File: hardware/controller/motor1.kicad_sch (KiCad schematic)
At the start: 55 parts, among them J10 Conn_01x01, J11 Conn_01x01, J12 Conn_02x03_Odd_Even, J9 Conn_01x01, Q10 AOD66406, Q11 AOD66406, Q12 AOD66406, Q13 AOD66406, Q8 AOD66406, Q9 AOD66406, U14 LM2105D, U15 MCP6541, U16 LM2105D, U17 MCP6541, U18 LM2105D, U19 MCP6541

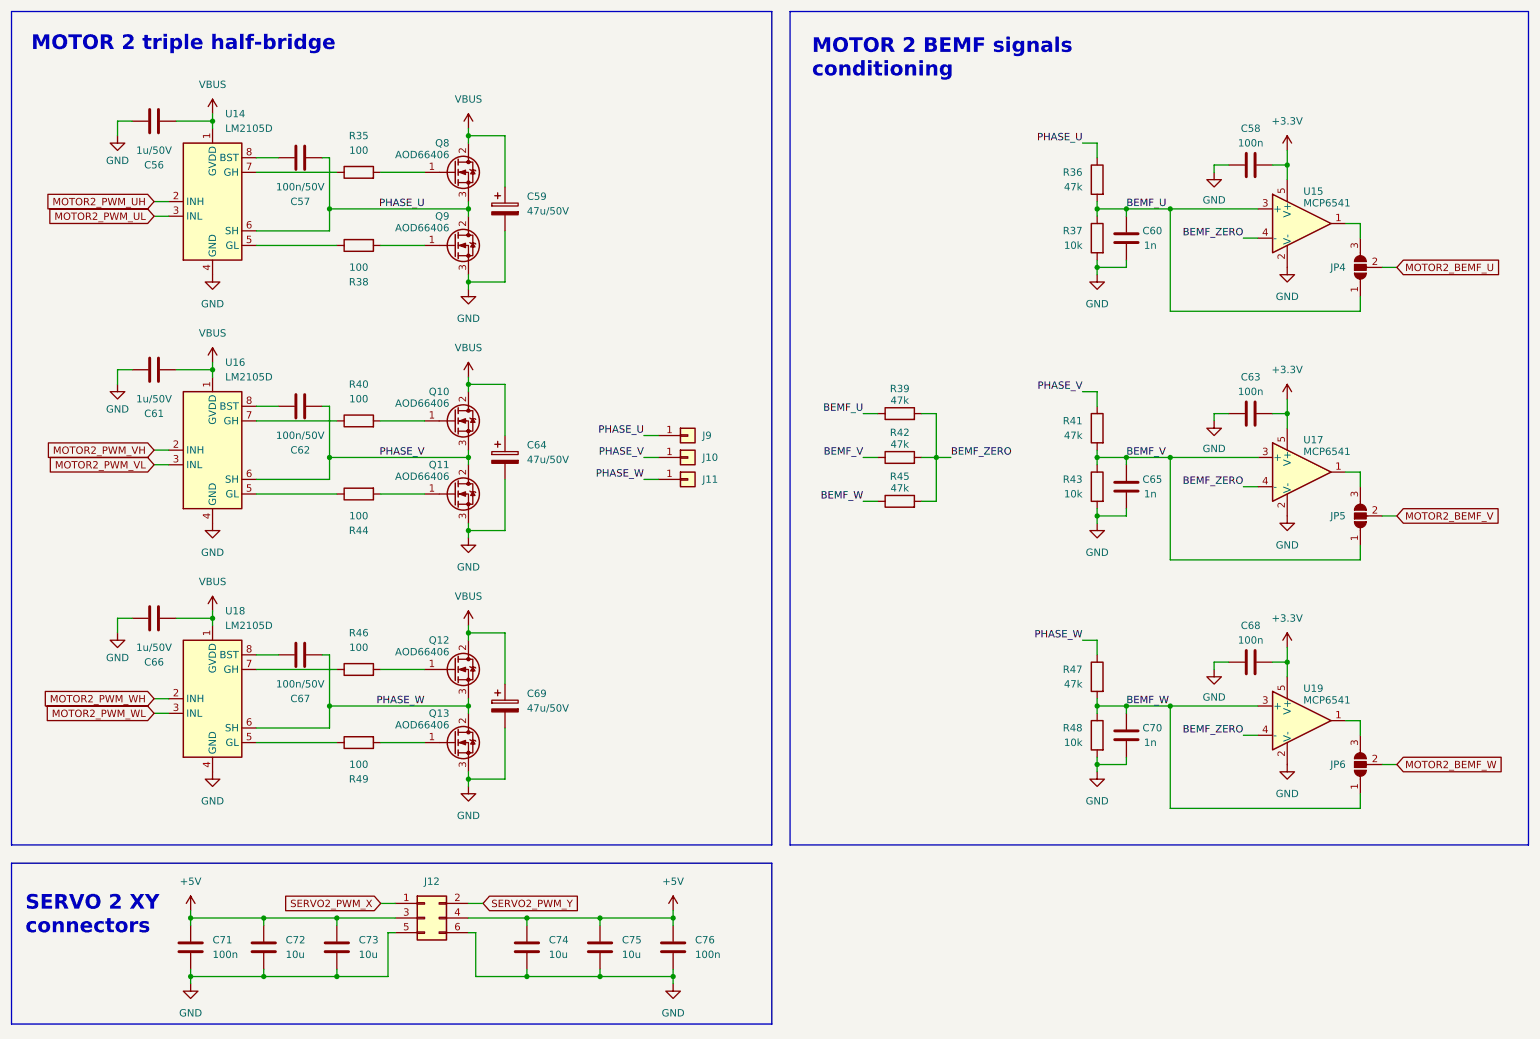
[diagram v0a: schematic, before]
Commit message: wip
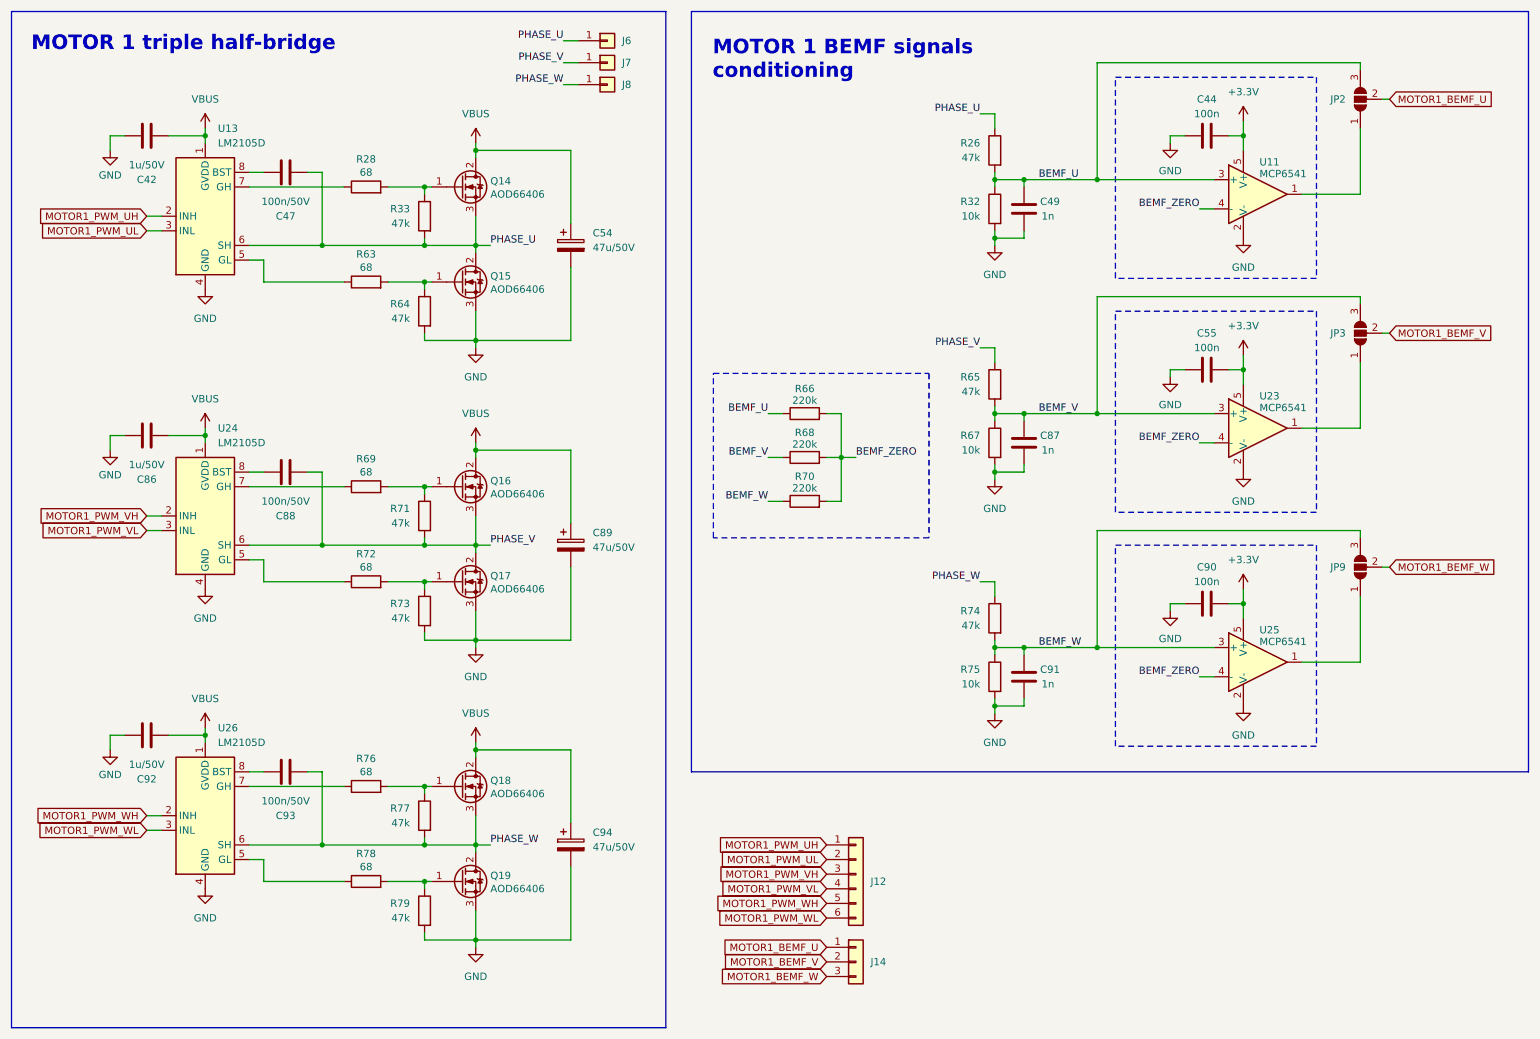
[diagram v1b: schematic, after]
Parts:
- removed C56, C61, C66: 1u/50V, Capacitor_SMD:C_0603_1608Metric, symbol Device:C
- removed C57, C62, C67: 100n/50V, Capacitor_SMD:C_0603_1608Metric, symbol Device:C
- removed C58, C63, C68, C71, C76: 100n, Capacitor_SMD:C_0603_1608Metric, symbol Device:C
- removed C59, C64, C69: 47u/50V, Capacitor_SMD:CP_Elec_6.3x7.7, symbol Device:C_Polarized
- removed C60, C65, C70: 1n, Capacitor_SMD:C_0603_1608Metric, symbol Device:C
- removed C72, C73, C74, C75: 10u, Capacitor_SMD:C_0603_1608Metric, symbol Device:C
- removed J10, J11, J9: Conn_01x01, Connector_Wire:SolderWire-2.5sqmm_1x01_D2.4mm_OD4.4mm, symbol Connector_Generic:Conn_01x01
- removed J12: Conn_02x03_Odd_Even, Connector_PinHeader_2.54mm:PinHeader_2x03_P2.54mm_Horizontal, symbol Connector_Generic:Conn_02x03_Odd_Even
- removed JP4, JP5, JP6: SolderJumper_3_Open, Jumper:SolderJumper-3_P1.3mm_Open_RoundedPad1.0x1.5mm, symbol Jumper:SolderJumper_3_Open
- removed Q10, Q11, Q12, Q13, Q8, Q9: AOD66406, Package_TO_SOT_SMD:TO-252-2, symbol Device:Q_NMOS_GDS
- removed R35, R38, R40, R44, R46, R49: 100, Resistor_SMD:R_0603_1608Metric, symbol Device:R
- removed R36, R39, R41, R42, R45, R47: 47k, Resistor_SMD:R_0603_1608Metric, symbol Device:R
- removed R37, R43, R48: 10k, Resistor_SMD:R_0603_1608Metric, symbol Device:R
- removed U14, U16, U18: LM2105D, Package_SO:SOIC-8_3.9x4.9mm_P1.27mm, symbol Driver_FET:LM2105D
- removed U15, U17, U19: MCP6541, Package_TO_SOT_SMD:SOT-23-5, symbol Comparator:MCP6561-OT
- added C42, C86, C92: 1u/50V, Capacitor_SMD:C_0603_1608Metric, symbol Device:C
- added C44, C55, C90: 100n, Capacitor_SMD:C_0603_1608Metric, symbol Device:C
- added C47, C88, C93: 100n/50V, Capacitor_SMD:C_0603_1608Metric, symbol Device:C
- added C49, C87, C91: 1n, Capacitor_SMD:C_0603_1608Metric, symbol Device:C
- added C54, C89, C94: 47u/50V, Capacitor_SMD:CP_Elec_6.3x7.7, symbol Device:C_Polarized
- added J12: Conn_01x06, symbol Connector_Generic:Conn_01x06
- added J14: Conn_01x03, symbol Connector_Generic:Conn_01x03
- added J6, J7, J8: Conn_01x01, Connector_Wire:SolderWire-2.5sqmm_1x01_D2.4mm_OD4.4mm, symbol Connector_Generic:Conn_01x01
- added JP2, JP3, JP9: SolderJumper_3_Open, Jumper:SolderJumper-3_P1.3mm_Open_RoundedPad1.0x1.5mm, symbol Jumper:SolderJumper_3_Open
- added Q14, Q15, Q16, Q17, Q18, Q19: AOD66406, Package_TO_SOT_SMD:TO-252-2, symbol Device:Q_NMOS_GDS
- added R26, R33, R64, R65, R71, R73, R74, R77, R79: 47k, Resistor_SMD:R_0603_1608Metric, symbol Device:R
- added R28, R63, R69, R72, R76, R78: 68, Resistor_SMD:R_0603_1608Metric, symbol Device:R
- added R32, R67, R75: 10k, Resistor_SMD:R_0603_1608Metric, symbol Device:R
- added R66, R68, R70: 220k, Resistor_SMD:R_0603_1608Metric, symbol Device:R
- added U11, U23, U25: MCP6541, Package_TO_SOT_SMD:SOT-23-5, symbol Comparator:MCP6561-OT
- added U13, U24, U26: LM2105D, Package_SO:SOIC-8_3.9x4.9mm_P1.27mm, symbol Driver_FET:LM2105D
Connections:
- net +3.3V: now also C44.2, C55.2, C90.2, U11.5 (V+), U23.5 (V+), U25.5 (V+)
- net BEMF_U: now also C49.1, JP2.3 (B), R26.2, R32.1, R66.1, U11.3 (+)
- net BEMF_V: now also C87.1, JP3.3 (B), R65.2, R67.1, R68.1, U23.3 (+)
- net BEMF_W: now also C91.1, JP9.3 (B), R70.1, R74.2, R75.1, U25.3 (+)
- net BEMF_ZERO: now also R66.2, R68.2, R70.2, U11.4 (-), U23.4 (-), U25.4 (-)
- net GND: now also C42.1, C44.1, C49.2, C54.2, C55.1, C86.1, C87.2, C89.2, C90.1, C91.2, C92.1, C94.2, Q15.3 (S), Q17.3 (S), Q19.3 (S), R32.2, R64.2, R67.2, R73.2, R75.2, R79.2, U11.2 (V-), U13.4 (GND), U23.2 (V-), U24.4 (GND), U25.2 (V-), U26.4 (GND)
- net PHASE_U: now also C47.2, J6.1 (Pin_1), Q14.3 (S), Q15.2 (D), R26.1, R33.2, U13.6 (SH)
- net PHASE_V: now also C88.2, J7.1 (Pin_1), Q16.3 (S), Q17.2 (D), R65.1, R71.2, U24.6 (SH)
- net PHASE_W: now also C93.2, J8.1 (Pin_1), Q18.3 (S), Q19.2 (D), R74.1, R77.2, U26.6 (SH)
- net VBUS: now also C42.2, C54.1, C86.2, C89.1, C92.2, C94.1, Q14.2 (D), Q16.2 (D), Q18.2 (D), U13.1 (GVDD), U24.1 (GVDD), U26.1 (GVDD)
- new net: Q19.1 (G), R78.2, R79.1
- new net: Q16.1 (G), R69.2, R71.1
- new net: R63.1, U13.5 (GL)
- new net: R28.1, U13.7 (GH)
- new net: C47.1, U13.8 (BST)
- new net: R72.1, U24.5 (GL)
- new net: R69.1, U24.7 (GH)
- new net: C88.1, U24.8 (BST)
- new net: Q15.1 (G), R63.2, R64.1
- new net: Q17.1 (G), R72.2, R73.1
- new net: C93.1, U26.8 (BST)
- new net: Q18.1 (G), R76.2, R77.1
- new net: R78.1, U26.5 (GL)
- new net: JP2.1 (A), U11.1
- new net: R76.1, U26.7 (GH)
- new net: JP3.1 (A), U23.1
- new net: Q14.1 (G), R28.2, R33.1
- new net: JP9.1 (A), U25.1
- new net MOTOR1_BEMF_U: J14.1 (Pin_1), JP2.2 (C)
- new net MOTOR1_BEMF_V: J14.2 (Pin_2), JP3.2 (C)
- new net MOTOR1_BEMF_W: J14.3 (Pin_3), JP9.2 (C)
- new net MOTOR1_PWM_UH: J12.1 (Pin_1), U13.2 (INH)
- new net MOTOR1_PWM_UL: J12.2 (Pin_2), U13.3 (INL)
- new net MOTOR1_PWM_VH: J12.3 (Pin_3), U24.2 (INH)
- new net MOTOR1_PWM_VL: J12.4 (Pin_4), U24.3 (INL)
- new net MOTOR1_PWM_WH: J12.5 (Pin_5), U26.2 (INH)
- new net MOTOR1_PWM_WL: J12.6 (Pin_6), U26.3 (INL)
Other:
- note added: "MOTOR 1 BEMF signals conditioning"
- note added: "MOTOR 1 triple half-bridge"
- note removed: "MOTOR 2 BEMF signals conditioning"
- note removed: "MOTOR 2 triple half-bridge"
- note removed: "SERVO 2 XY connectors"
